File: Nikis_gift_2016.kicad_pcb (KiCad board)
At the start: 2 copper layers, 32 parts, among them CON1 BARREL_JACK, IC1 ATMEGA328P-A, P1 CONN_01X06, SW1 SW_PUSH, SW2 SW_PUSH, SW3 SW_PUSH, SW4 SW_PUSH, SW5 SW_PUSH, U1 LM7805CT, U2 DS1338

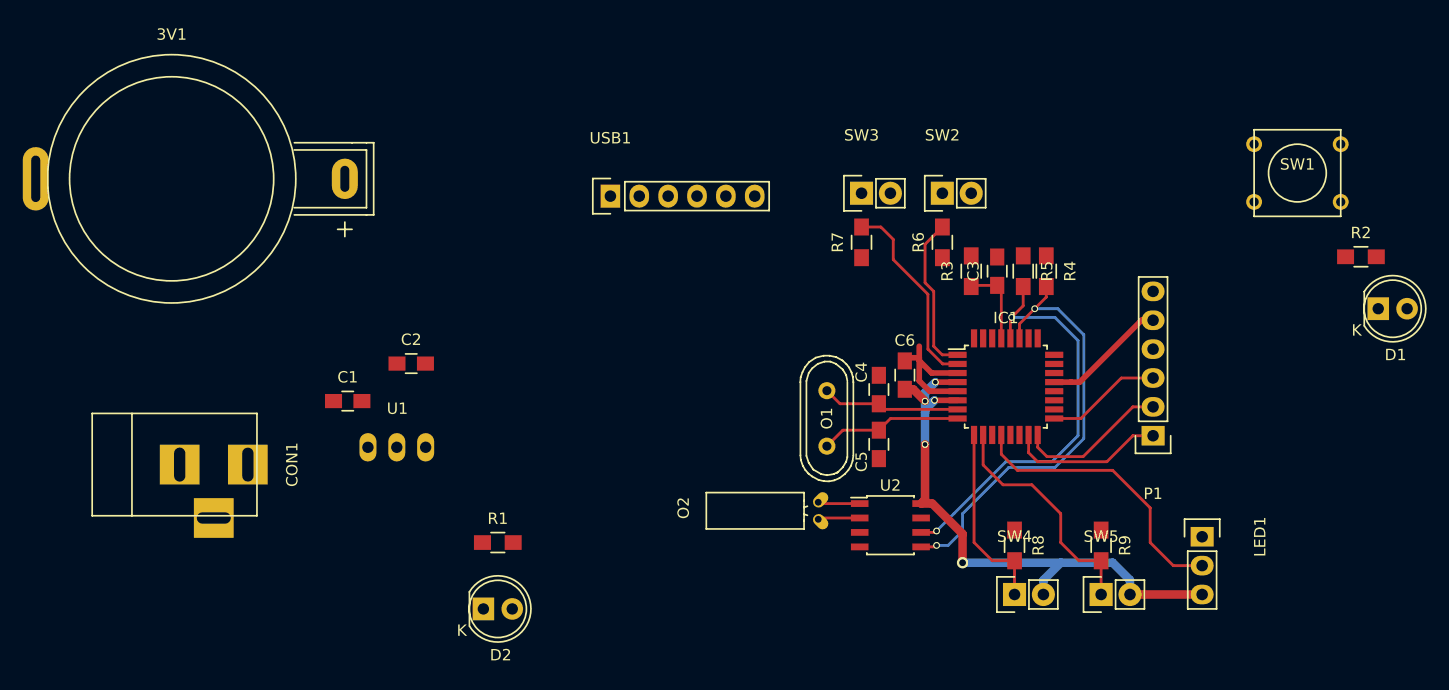
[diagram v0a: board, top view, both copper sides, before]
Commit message: gerber
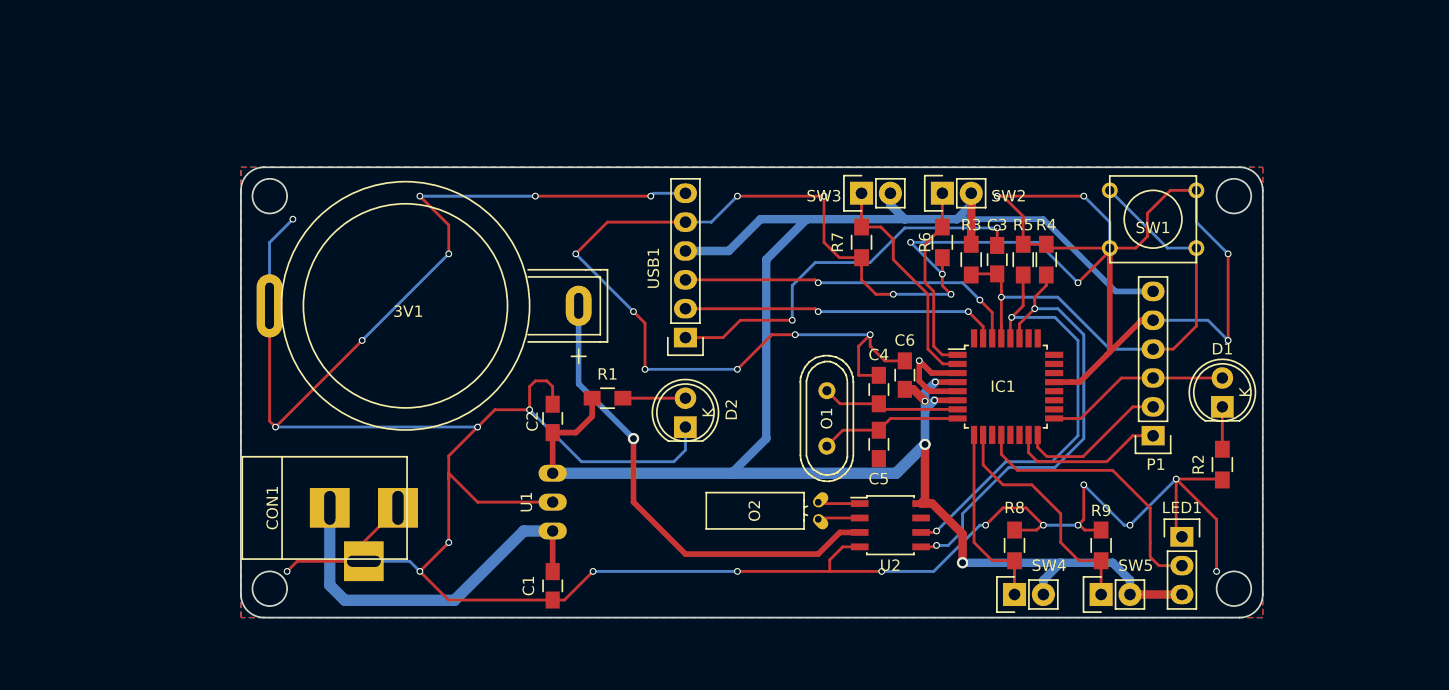
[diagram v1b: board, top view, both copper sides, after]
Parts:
- SW1: footprint Buttons_Switches_ThroughHole:SW_PUSH_SMALL -> KiCAD_Lib:SW_PUSH_SMALL-diag
- moved C1 24.3 mm to (105.7, 115.6), turned to 90 degrees
- moved D2 23.9 mm to (117.3, 101.6), turned to 90 degrees
- moved 3V1 23.4 mm to (108.0, 90.9)
- moved R2 22.0 mm to (164.6, 104.9), turned to 90 degrees
- moved D1 16.2 mm to (164.6, 99.8), turned to 90 degrees
- moved R1 16.0 mm to (110.5, 99.1)
- moved U1 14.5 mm to (105.7, 108.2), turned to 90 degrees
- moved USB1 14.1 mm to (117.3, 93.7), turned to 90 degrees
- moved CON1 13.7 mm to (85.9, 108.7)
- moved C2 13.3 mm to (105.7, 100.8), turned to 270 degrees
- moved SW1 13.3 mm to (158.5, 83.3), turned to 180 degrees
- moved LED1 1.78 mm to (161.0, 111.3)
- moved C3 1.02 mm to (144.8, 86.9)
- moved R3 1.02 mm to (142.5, 86.9)
- moved R4 1.02 mm to (149.1, 86.9)
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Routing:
- net GND: track 23.0 -> 471.0 mm, vias 0 -> 40
- net +5V: track 52.3 -> 173.7 mm
- net Net-(3V1-Pad1): track 0.00 -> 41.9 mm, vias 0 -> 1
- net Net-(C3-Pad1): track 7.14 -> 44.7 mm, vias 0 -> 1
- net Net-(C3-Pad2): track 0.00 -> 34.8 mm, vias 0 -> 2
- net Net-(C1-Pad2): track 0.00 -> 33.1 mm
- net Net-(IC1-Pad30): track 0.00 -> 30.5 mm, vias 0 -> 2
- net Net-(IC1-Pad31): track 0.00 -> 27.9 mm, vias 0 -> 2
- net Net-(D1-Pad2): track 10.2 -> 16.3 mm
- net Net-(D2-Pad2): track 0.00 -> 5.51 mm
- net Net-(D1-Pad1): track 0.00 -> 3.73 mm
- net Net-(IC1-Pad2): track 17.3 -> 20.3 mm
- net Net-(IC1-Pad1): track 13.9 -> 16.8 mm
- net Net-(IC1-Pad12): track 25.2 -> 24.2 mm
- net Net-(IC1-Pad28): track 37.6 -> 38.6 mm
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- added copper zone on B.Cu, net GND
- added copper zone on F.Cu, net GND
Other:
- board outline added: 89.9 x 39.6 mm
- rule pad_to_mask_clearance: 0.2 -> -0.125
